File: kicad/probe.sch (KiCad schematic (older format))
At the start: 15 parts, among them IC1 ATTINY85, IC2 MAX7219, P2 5V

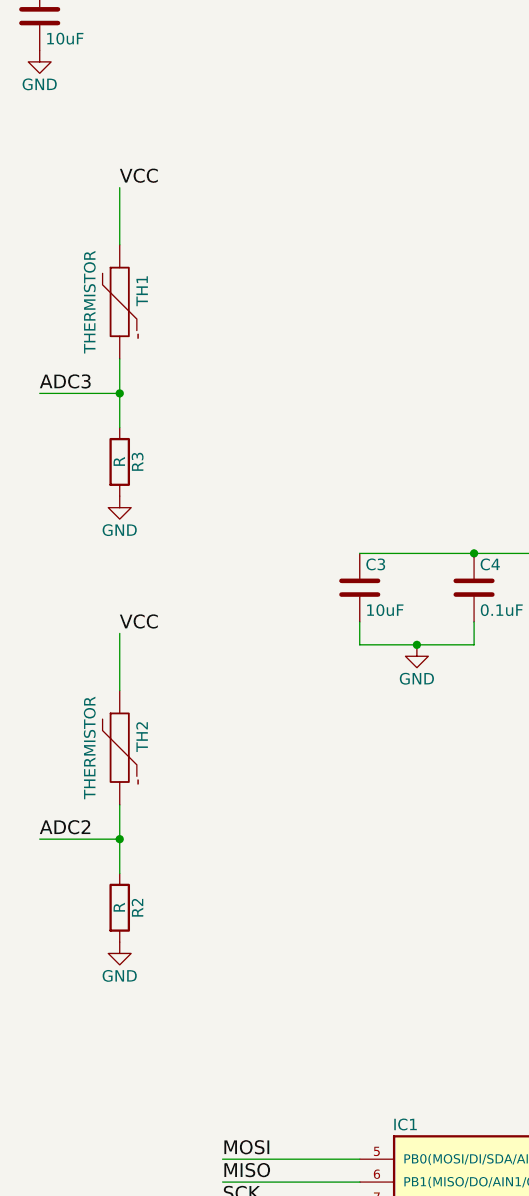
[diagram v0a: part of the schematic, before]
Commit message: Better accuracy
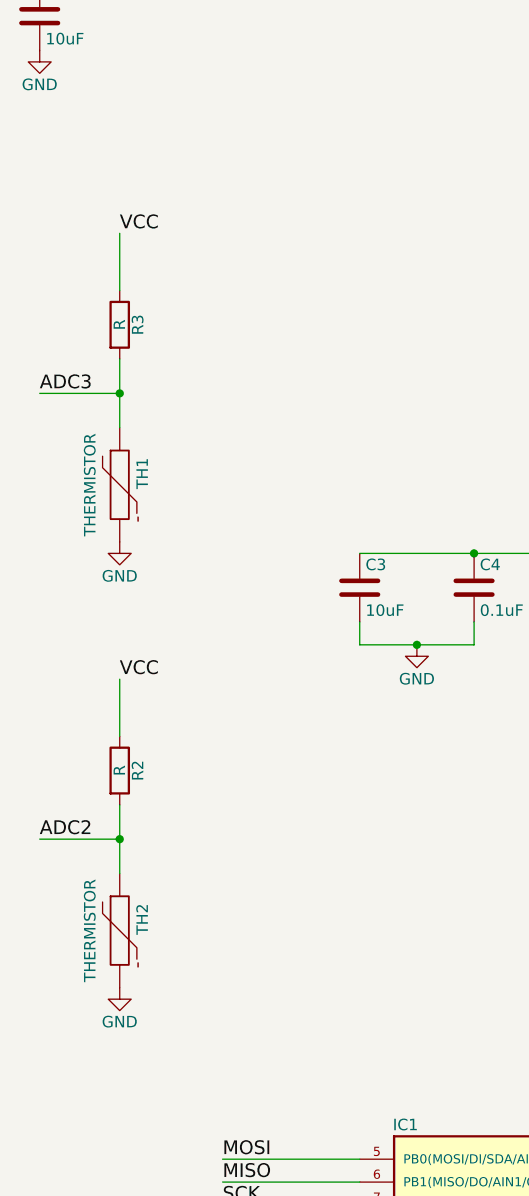
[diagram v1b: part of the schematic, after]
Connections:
- net ADC2: now also R2.2, TH2.1; no longer R2.1, TH2.2
- net ADC3: now also R3.2, TH1.1; no longer R3.1, TH1.2
- net GND: now also TH1.2, TH2.2; no longer R2.2, R3.2
- net VCC: now also R2.1, R3.1; no longer TH1.1, TH2.1
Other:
- moved on the sheet: R2, R3, TH1, TH2
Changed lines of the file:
@@
 L THERMISTOR TH1
 U 1 1 57D69809
-P 1400 2400
-F 0 "TH1" V 1500 2450 50  0000 C CNN
-F 1 "THERMISTOR" V 1300 2400 50  0000 C BNN
-F 2 "Discret:R1" H 1400 2400 50  0001 C CNN
-F 3 "" H 1400 2400 50  0000 C CNN
-	1    1400 2400
+P 1400 3200
+F 0 "TH1" V 1500 3250 50  0000 C CNN
+F 1 "THERMISTOR" V 1300 3200 50  0000 C BNN
+F 2 "Discret:R1" H 1400 3200 50  0001 C CNN
+F 3 "" H 1400 3200 50  0000 C CNN
+	1    1400 3200
 	1    0    0    -1
 $EndComp
@@
 L R R3
 U 1 1 57D698E5
-P 1400 3100
-F 0 "R3" V 1480 3100 50  0000 C CNN
-F 1 "R" V 1400 3100 50  0000 C CNN
-F 2 "Resistors_SMD:R_0805_HandSoldering" V 1330 3100 50  0001 C CNN
-F 3 "" H 1400 3100 50  0000 C CNN
-	1    1400 3100
+P 1400 2500
+F 0 "R3" V 1480 2500 50  0000 C CNN
+F 1 "R" V 1400 2500 50  0000 C CNN
+F 2 "Resistors_SMD:R_0805_HandSoldering" V 1330 2500 50  0001 C CNN
+F 3 "" H 1400 2500 50  0000 C CNN
+	1    1400 2500
 	1    0    0    -1
 $EndComp
@@
 L GND #PWR2
 U 1 1 57D6D625
-P 1400 3250
-F 0 "#PWR2" H 1400 3000 50  0001 C CNN
-F 1 "GND" H 1400 3100 50  0000 C CNN
-F 2 "" H 1400 3250 50  0000 C CNN
-F 3 "" H 1400 3250 50  0000 C CNN
-	1    1400 3250
+P 1400 3450
+F 0 "#PWR2" H 1400 3200 50  0001 C CNN
+F 1 "GND" H 1400 3300 50  0000 C CNN
+F 2 "" H 1400 3450 50  0000 C CNN
+F 3 "" H 1400 3450 50  0000 C CNN
+	1    1400 3450
 	1    0    0    -1
 $EndComp
@@
 Wire Wire Line
 	1050 2800 1400 2800
-Text Label 1400 1900 0    60   ~ 0
-VCC
-Wire Wire Line
-	1400 1900 1400 2150
+Text Label 1400 2100 0    60   ~ 0
+VCC
+Wire Wire Line
+	1400 2100 1400 2350
 Text Label 3450 3500 0    60   ~ 0
 VCC
@@
 L THERMISTOR TH2
 U 1 1 57DEB3C1
-P 1400 4350
-F 0 "TH2" V 1500 4400 50  0000 C CNN
-F 1 "THERMISTOR" V 1300 4350 50  0000 C BNN
-F 2 "Discret:R1" H 1400 4350 50  0001 C CNN
-F 3 "" H 1400 4350 50  0000 C CNN
-	1    1400 4350
+P 1400 5150
+F 0 "TH2" V 1500 5200 50  0000 C CNN
+F 1 "THERMISTOR" V 1300 5150 50  0000 C BNN
+F 2 "Discret:R1" H 1400 5150 50  0001 C CNN
+F 3 "" H 1400 5150 50  0000 C CNN
+	1    1400 5150
 	1    0    0    -1
 $EndComp
@@
 L R R2
 U 1 1 57DEB3C7
-P 1400 5050
-F 0 "R2" V 1480 5050 50  0000 C CNN
-F 1 "R" V 1400 5050 50  0000 C CNN
-F 2 "Resistors_SMD:R_0805_HandSoldering" V 1330 5050 50  0001 C CNN
-F 3 "" H 1400 5050 50  0000 C CNN
-	1    1400 5050
+P 1400 4450
+F 0 "R2" V 1480 4450 50  0000 C CNN
+F 1 "R" V 1400 4450 50  0000 C CNN
+F 2 "Resistors_SMD:R_0805_HandSoldering" V 1330 4450 50  0001 C CNN
+F 3 "" H 1400 4450 50  0000 C CNN
+	1    1400 4450
 	1    0    0    -1
 $EndComp
@@
 L GND #PWR3
 U 1 1 57DEB3CD
-P 1400 5200
-F 0 "#PWR3" H 1400 4950 50  0001 C CNN
-F 1 "GND" H 1400 5050 50  0000 C CNN
-F 2 "" H 1400 5200 50  0000 C CNN
-F 3 "" H 1400 5200 50  0000 C CNN
-	1    1400 5200
+P 1400 5400
+F 0 "#PWR3" H 1400 5150 50  0001 C CNN
+F 1 "GND" H 1400 5250 50  0000 C CNN
+F 2 "" H 1400 5400 50  0000 C CNN
+F 3 "" H 1400 5400 50  0000 C CNN
+	1    1400 5400
 	1    0    0    -1
 $EndComp
@@
 Wire Wire Line
 	1050 4750 1400 4750
-Text Label 1400 3850 0    60   ~ 0
-VCC
-Wire Wire Line
-	1400 3850 1400 4100
+Text Label 1400 4050 0    60   ~ 0
+VCC
+Wire Wire Line
+	1400 4050 1400 4300
 Text Label 3550 4800 0    60   ~ 0
 MISO
